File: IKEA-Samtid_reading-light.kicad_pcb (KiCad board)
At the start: 2 copper layers, 21 x 100 mm, 30 parts, among them IC1 ATTINY25-S, P1 CONN_2, U1 MCP1804-SOT23-5, U2 PT4115-SOT89-5

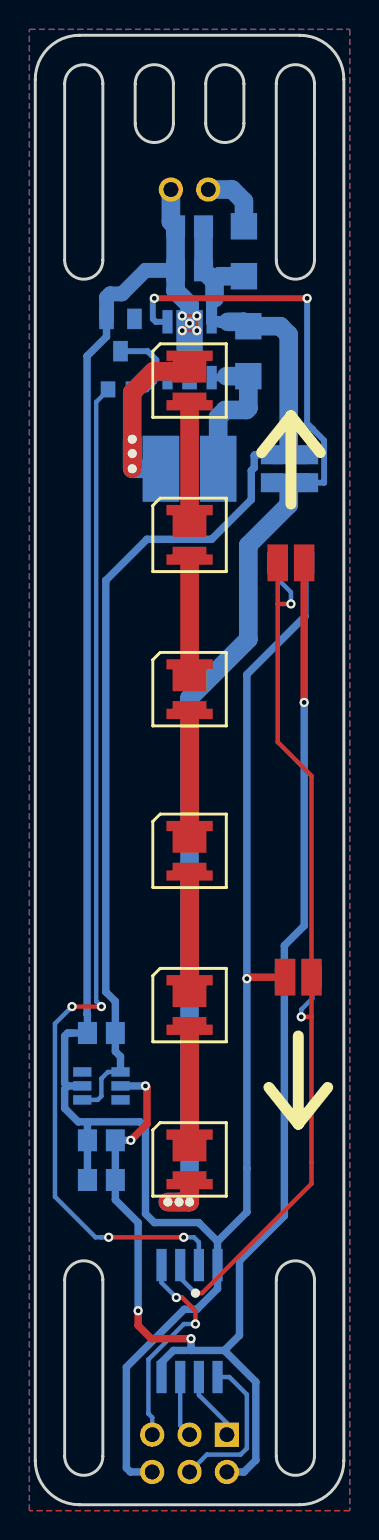
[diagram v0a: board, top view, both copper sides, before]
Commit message: Shoved parts around a bit. Visually more pleasing now.
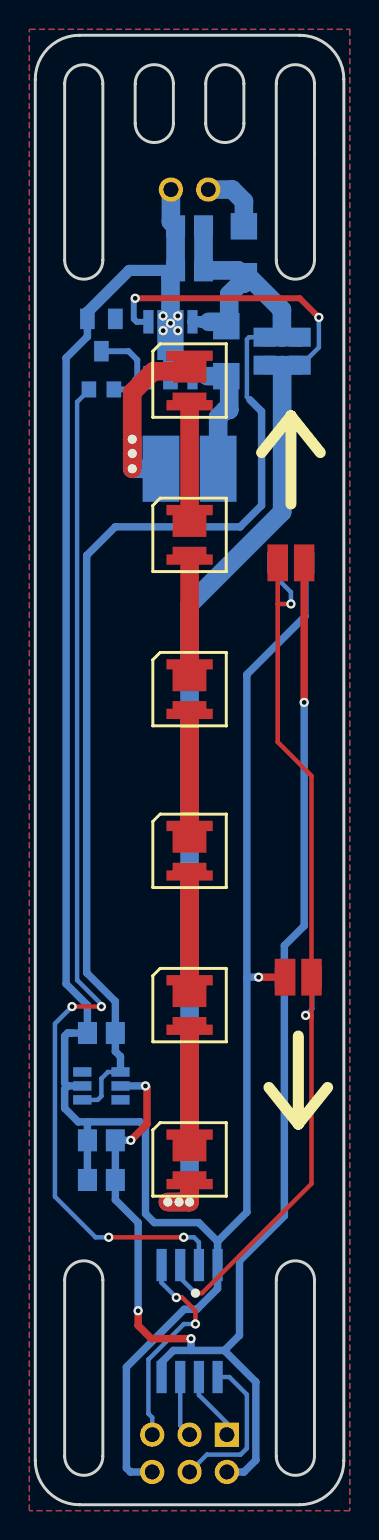
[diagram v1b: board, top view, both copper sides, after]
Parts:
- moved R_CS1 8.02 mm to (78.5, 60.0)
- moved R_CS2 8.02 mm to (76.1, 60.0)
- moved DS2 1.50 mm to (73.5, 60.0)
- moved DZ1 1.30 mm to (65.0, 58.9)
- moved R2 1.30 mm to (65.0, 62.6)
- moved U2 1.30 mm to (69.7, 59.9)
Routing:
- net +24V: track 79.7 -> 86.8 mm
- net GNDPWR: track 75.9 -> 70.9 mm
- net /SW: track 10.5 -> 9.31 mm
- net /DIM: track 70.5 -> 71.1 mm
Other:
- board text added: "2014 - blog.spitzenpfeil.org Reading-light I**A S*mt*d V0.10.a"
- board text removed: "2014 - blog.spitzenpfeil.org Reading-light I**A S*mt*d"
